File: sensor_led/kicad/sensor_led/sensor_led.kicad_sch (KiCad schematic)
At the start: 5 parts

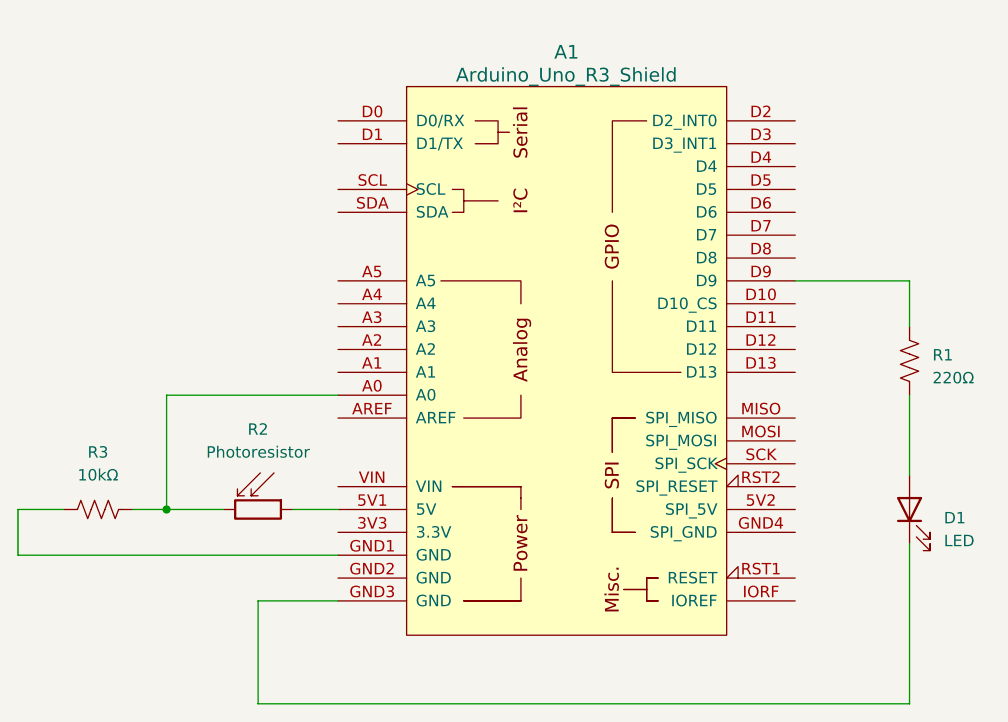
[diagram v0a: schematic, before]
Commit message: Use default Arduino UNO R3 symbol
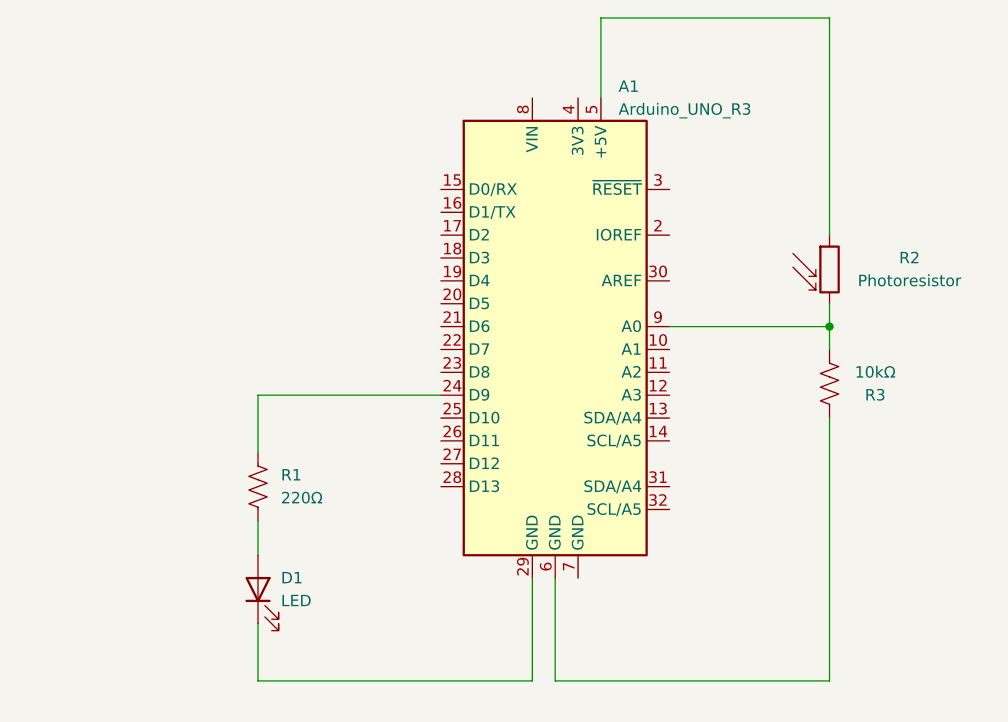
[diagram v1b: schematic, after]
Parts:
- removed A1: Arduino_Uno_R3_Shield, PCM_arduino-library:Arduino_Uno_R3_Shield, symbol PCM_arduino-library:Arduino_Uno_R3_Shield
- added A1: Arduino_UNO_R3, Module:Arduino_UNO_R3, symbol MCU_Module:Arduino_UNO_R3
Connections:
- net at R2.1: now also A1.5 (+5V)
- net at R3.1: now also A1.6 (GND); no longer R2.2
- net at R1.1: now also A1.24 (D9)
- net at R3.2: now also R2.2, A1.9 (A0)
- net at D1.1 (K): now also A1.29 (GND)
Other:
- moved on the sheet: D1, R1, R2, R3
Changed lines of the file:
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@@
     (title "Sensor LED")
   )
-  (junction (at 57.15 74.93) (diameter 0) (color 0 0 0 0)
+  (junction (at 130.81 54.61) (diameter 0) (color 0 0 0 0)
   )
-  (wire (pts (xy 53.34 74.93) (xy 57.15 74.93))
+  (wire (pts (xy 100.33 93.98) (xy 100.33 82.55))
     (stroke (width 0) (type default))
   )
-  (wire (pts (xy 127 49.53) (xy 139.7 49.53))
+  (wire (pts (xy 105.41 29.21) (xy 105.41 20.32))
     (stroke (width 0) (type default))
   )
-  (wire (pts (xy 139.7 49.53) (xy 139.7 54.61))
+  (wire (pts (xy 67.31 76.2) (xy 67.31 80.01))
     (stroke (width 0) (type default))
   )
-  (wire (pts (xy 67.31 96.52) (xy 67.31 85.09))
+  (wire (pts (xy 105.41 20.32) (xy 130.81 20.32))
     (stroke (width 0) (type default))
   )
-  (wire (pts (xy 139.7 96.52) (xy 67.31 96.52))
+  (wire (pts (xy 87.63 62.23) (xy 67.31 62.23))
     (stroke (width 0) (type default))
   )
-  (wire (pts (xy 40.64 74.93) (xy 40.64 80.01))
+  (wire (pts (xy 130.81 52.07) (xy 130.81 54.61))
     (stroke (width 0) (type default))
   )
-  (wire (pts (xy 40.64 80.01) (xy 76.2 80.01))
+  (wire (pts (xy 130.81 20.32) (xy 130.81 44.45))
     (stroke (width 0) (type default))
   )
-  (wire (pts (xy 139.7 62.23) (xy 139.7 71.12))
+  (wire (pts (xy 130.81 54.61) (xy 113.03 54.61))
     (stroke (width 0) (type default))
   )
-  (wire (pts (xy 71.12 74.93) (xy 76.2 74.93))
+  (wire (pts (xy 67.31 62.23) (xy 67.31 68.58))
     (stroke (width 0) (type default))
   )
-  (wire (pts (xy 57.15 74.93) (xy 63.5 74.93))
+  (wire (pts (xy 67.31 93.98) (xy 97.79 93.98))
     (stroke (width 0) (type default))
   )
-  (wire (pts (xy 139.7 78.74) (xy 139.7 96.52))
+  (wire (pts (xy 67.31 87.63) (xy 67.31 93.98))
     (stroke (width 0) (type default))
   )
-  (wire (pts (xy 57.15 74.93) (xy 57.15 62.23))
+  (wire (pts (xy 97.79 93.98) (xy 97.79 82.55))
     (stroke (width 0) (type default))
   )
-  (wire (pts (xy 57.15 62.23) (xy 76.2 62.23))
+  (wire (pts (xy 130.81 93.98) (xy 100.33 93.98))
     (stroke (width 0) (type default))
   )
-  (wire (pts (xy 45.72 74.93) (xy 40.64 74.93))
+  (wire (pts (xy 130.81 64.77) (xy 130.81 93.98))
     (stroke (width 0) (type default))
   )
-  (wire (pts (xy 67.31 85.09) (xy 76.2 85.09))
+  (wire (pts (xy 130.81 54.61) (xy 130.81 57.15))
     (stroke (width 0) (type default))
   )
-  (symbol (lib_id "PCM_arduino-library:Arduino_Uno_R3_Shield") (at 101.6 58.42 0) (unit 1)
-    (in_bom yes) (on_board yes) (dnp no) (fields_autoplaced)
-    (property "Reference" "A1" (at 101.6 24.13 0)
-      (effects (font (size 1.524 1.524)))
-    )
-    (property "Value" "Arduino_Uno_R3_Shield" (at 101.6 26.67 0)
-      (effects (font (size 1.524 1.524)))
-    )
-    (property "Footprint" "PCM_arduino-library:Arduino_Uno_R3_Shield" (at 101.6 96.52 0)
-      (effects (font (size 1.524 1.524)) hide)
-    )
-    (property "Datasheet" "https://docs.arduino.cc/hardware/uno-rev3" (at 101.6 92.71 0)
-      (effects (font (size 1.524 1.524)) hide)
-    )
-    (pin "3V3")
-    (pin "5V1")
-    (pin "5V2")
-    (pin "A0")
-    (pin "A1")
-    (pin "A2")
-    (pin "A3")
-    (pin "A4")
-    (pin "A5")
-    (pin "AREF")
-    (pin "D0")
-    (pin "D1")
-    (pin "D10")
-    (pin "D11")
-    (pin "D12")
-    (pin "D13")
-    (pin "D2")
-    (pin "D3")
-    (pin "D4")
-    (pin "D5")
-    (pin "D6")
-    (pin "D7")
-    (pin "D8")
-    (pin "D9")
-    (pin "GND1")
-    (pin "GND2")
-    (pin "GND3")
-    (pin "GND4")
-    (pin "IORF")
-    (pin "MISO")
-    (pin "MOSI")
-    (pin "RST1")
-    (pin "RST2")
-    (pin "SCK")
-    (pin "SCL")
-    (pin "SDA")
-    (pin "VIN")
-    (instances
-      (project "sensor_led"
-        (path "/c28b344a-4fcb-4203-a01e-172d139c4367"
-          (reference "A1") (unit 1)
-        )
-      )
-    )
-  )
-  (symbol (lib_id "Device:LED") (at 139.7 74.93 90) (unit 1)
-    (in_bom yes) (on_board yes) (dnp no) (fields_autoplaced)
-    (property "Reference" "D1" (at 143.51 75.8825 90)
+  (symbol (lib_id "Device:LED") (at 67.31 83.82 90) (unit 1)
+    (in_bom yes) (on_board yes) (dnp no)
+    (property "Reference" "D1" (at 69.85 82.55 90)
       (effects (font (size 1.27 1.27)) (justify right))
     )
-    (property "Value" "LED" (at 143.51 78.4225 90)
+    (property "Value" "LED" (at 69.85 85.09 90)
       (effects (font (size 1.27 1.27)) (justify right))
     )
-    (property "Footprint" "" (at 139.7 74.93 0)
+    (property "Footprint" "" (at 67.31 83.82 0)
       (effects (font (size 1.27 1.27)) hide)
     )
-    (property "Datasheet" "~" (at 139.7 74.93 0)
+    (property "Datasheet" "~" (at 67.31 83.82 0)
       (effects (font (size 1.27 1.27)) hide)
     )
@@
     )
   )
-  (symbol (lib_id "Device:R_US") (at 49.53 74.93 270) (unit 1)
+  (symbol (lib_id "Device:R_US") (at 130.81 60.96 180) (unit 1)
     (in_bom yes) (on_board yes) (dnp no)
-    (property "Reference" "R3" (at 49.53 68.58 90)
+    (property "Reference" "R3" (at 135.89 62.23 0)
       (effects (font (size 1.27 1.27)))
     )
-    (property "Value" "10kΩ" (at 49.53 71.12 90)
+    (property "Value" "10kΩ" (at 135.89 59.69 0)
       (effects (font (size 1.27 1.27)))
     )
-    (property "Footprint" "" (at 49.276 75.946 90)
+    (property "Footprint" "" (at 129.794 60.706 90)
       (effects (font (size 1.27 1.27)) hide)
     )
-    (property "Datasheet" "~" (at 49.53 74.93 0)
+    (property "Datasheet" "~" (at 130.81 60.96 0)
       (effects (font (size 1.27 1.27)) hide)
     )
@@
     )
   )
-  (symbol (lib_id "Device:R_US") (at 139.7 58.42 0) (unit 1)
+  (symbol (lib_id "MCU_Module:Arduino_UNO_R3") (at 100.33 54.61 0) (unit 1)
     (in_bom yes) (on_board yes) (dnp no) (fields_autoplaced)
-    (property "Reference" "R1" (at 142.24 57.785 0)
+    (property "Reference" "A1" (at 107.3659 27.94 0)
       (effects (font (size 1.27 1.27)) (justify left))
     )
-    (property "Value" "220Ω" (at 142.24 60.325 0)
+    (property "Value" "Arduino_UNO_R3" (at 107.3659 30.48 0)
       (effects (font (size 1.27 1.27)) (justify left))
     )
-    (property "Footprint" "" (at 140.716 58.674 90)
+    (property "Footprint" "Module:Arduino_UNO_R3" (at 100.33 54.61 0)
+      (effects (font (size 1.27 1.27) italic) hide)
+    )
+    (property "Datasheet" "https://www.arduino.cc/en/Main/arduinoBoardUno" (at 100.33 54.61 0)
       (effects (font (size 1.27 1.27)) hide)
     )
-    (property "Datasheet" "~" (at 139.7 58.42 0)
+    (pin "1")
+    (pin "10")
+    (pin "11")
+    (pin "12")
+    (pin "13")
+    (pin "14")
+    (pin "15")
+    (pin "16")
+    (pin "17")
+    (pin "18")
+    (pin "19")
+    (pin "2")
+    (pin "20")
+    (pin "21")
+    (pin "22")
+    (pin "23")
+    (pin "24")
+    (pin "25")
+    (pin "26")
+    (pin "27")
+    (pin "28")
+    (pin "29")
+    (pin "3")
+    (pin "30")
+    (pin "31")
+    (pin "32")
+    (pin "4")
+    (pin "5")
+    (pin "6")
+    (pin "7")
+    (pin "8")
+    (pin "9")
+    (instances
+      (project "sensor_led"
+        (path "/c28b344a-4fcb-4203-a01e-172d139c4367"
+          (reference "A1") (unit 1)
+        )
+      )
+    )
+  )
+  (symbol (lib_id "Device:R_US") (at 67.31 72.39 0) (unit 1)
+    (in_bom yes) (on_board yes) (dnp no)
+    (property "Reference" "R1" (at 69.85 71.12 0)
+      (effects (font (size 1.27 1.27)) (justify left))
+    )
+    (property "Value" "220Ω" (at 69.85 73.66 0)
+      (effects (font (size 1.27 1.27)) (justify left))
+    )
+    (property "Footprint" "" (at 68.326 72.644 90)
+      (effects (font (size 1.27 1.27)) hide)
+    )
+    (property "Datasheet" "~" (at 67.31 72.39 0)
       (effects (font (size 1.27 1.27)) hide)
     )
@@
     )
   )
-  (symbol (lib_id "Device:R_Photo") (at 67.31 74.93 270) (unit 1)
+  (symbol (lib_id "Device:R_Photo") (at 130.81 48.26 0) (unit 1)
     (in_bom yes) (on_board yes) (dnp no)
-    (property "Reference" "R2" (at 67.31 66.04 90)
+    (property "Reference" "R2" (at 139.7 46.99 0)
       (effects (font (size 1.27 1.27)))
     )
-    (property "Value" "Photoresistor" (at 67.31 68.58 90)
+    (property "Value" "Photoresistor" (at 139.7 49.53 0)
       (effects (font (size 1.27 1.27)))
     )
-    (property "Footprint" "" (at 60.96 76.2 90)
+    (property "Footprint" "" (at 132.08 54.61 90)
       (effects (font (size 1.27 1.27)) (justify left) hide)
     )
-    (property "Datasheet" "~" (at 66.04 74.93 0)
+    (property "Datasheet" "~" (at 130.81 49.53 0)
       (effects (font (size 1.27 1.27)) hide)
     )
